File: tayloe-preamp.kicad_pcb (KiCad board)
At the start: 2 copper layers, 39 x 21 mm, 14 parts, among them J1 PCB_SMA_EDGE, J2 PCB_SMA_EDGE, J3 Conn_01x01_Female, Q1 2N2222

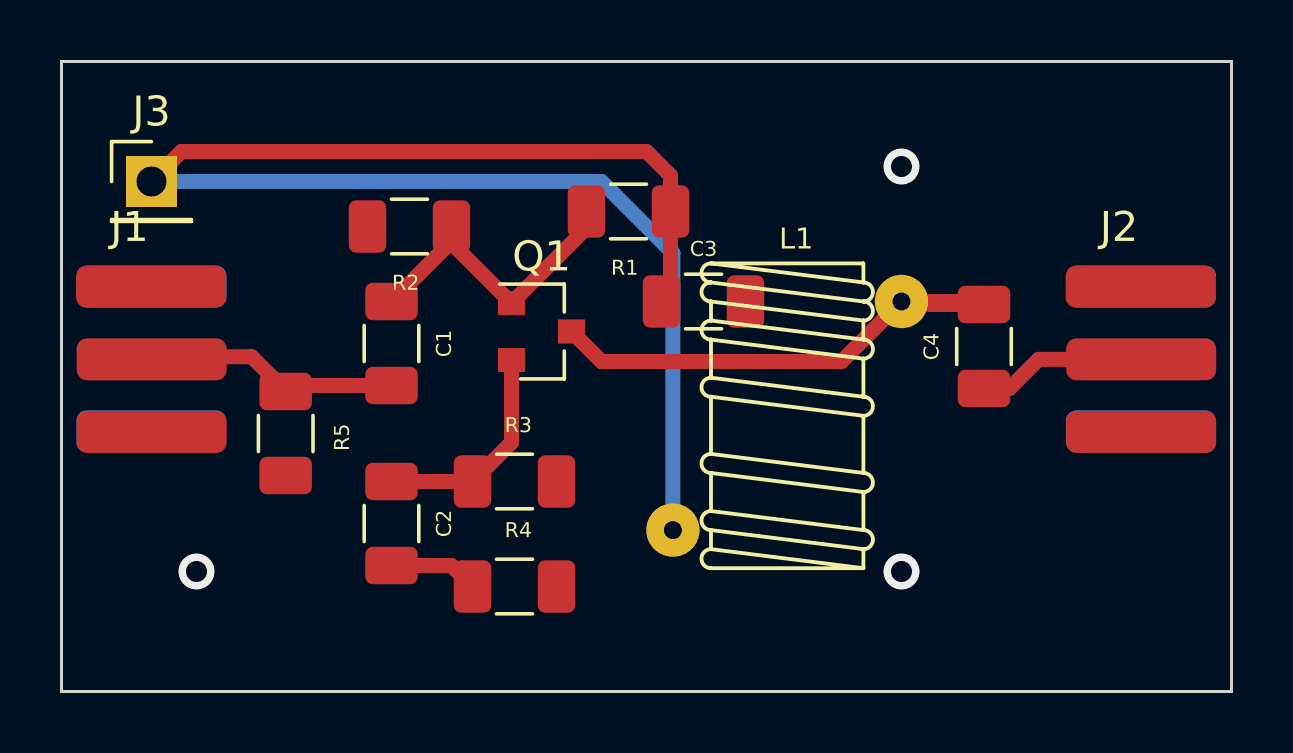
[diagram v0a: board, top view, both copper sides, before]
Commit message: gg
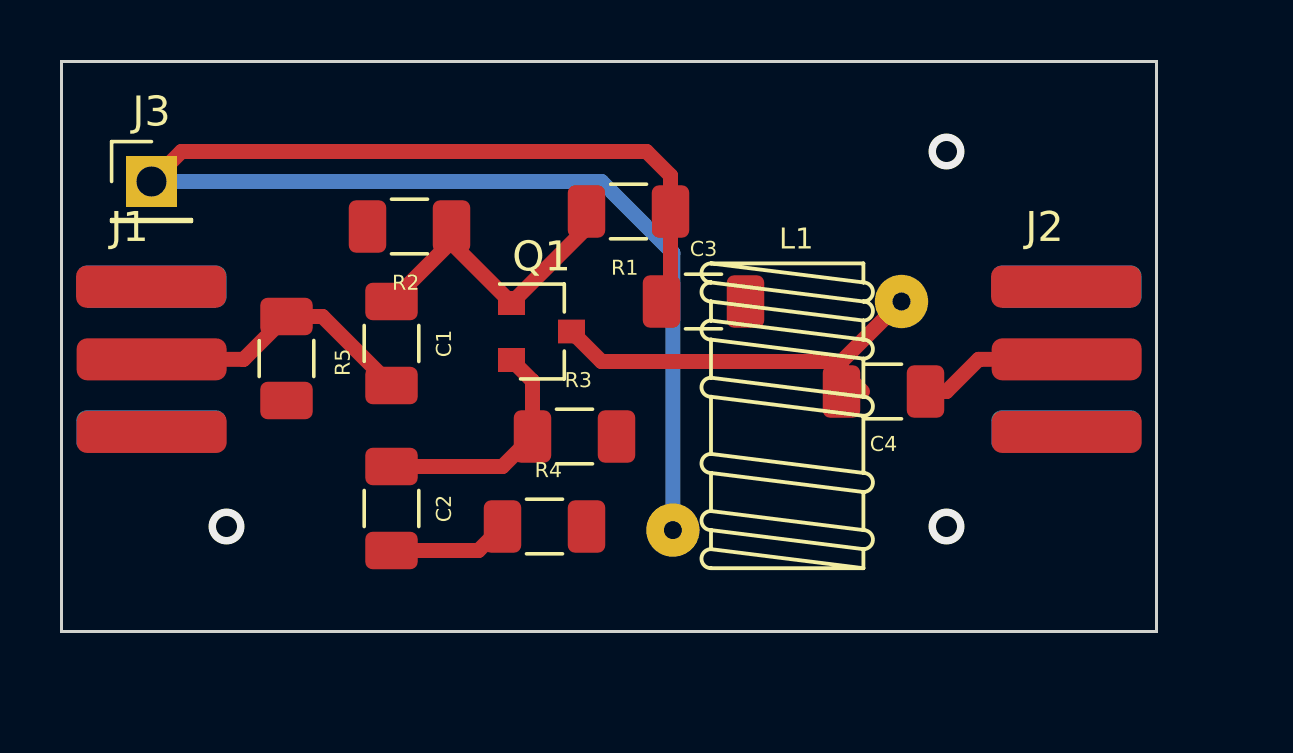
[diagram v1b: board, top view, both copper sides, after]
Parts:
- moved C4 3.91 mm to (171.4, 96.2), turned to 180 degrees
- moved R5 2.50 mm to (153.9, 93.0)
- moved R3 2.50 mm to (161.2, 93.1)
- moved J2 2.48 mm to (177.5, 87.8)
- moved R4 2.24 mm to (160.2, 96.1)
- moved C2 0.50 mm to (157.2, 97.9)
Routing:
- net Net-(C4-Pad2): track 16.9 -> 13.5 mm
- net Net-(C1-Pad2): track 8.39 -> 9.54 mm
- net Net-(C2-Pad2): track 2.99 -> 4.03 mm
- net Net-(C2-Pad1): track 7.29 -> 7.95 mm
- net Net-(C4-Pad1): track 5.65 -> 5.15 mm
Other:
- board size 39 x 21 mm -> 36.5 x 19 mm
